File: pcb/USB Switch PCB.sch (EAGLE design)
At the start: 25 parts, among them Q1 2N7002P, Q2 2N7002P, X1 AMPHENOL-0001LF, X2 UE27-USBA

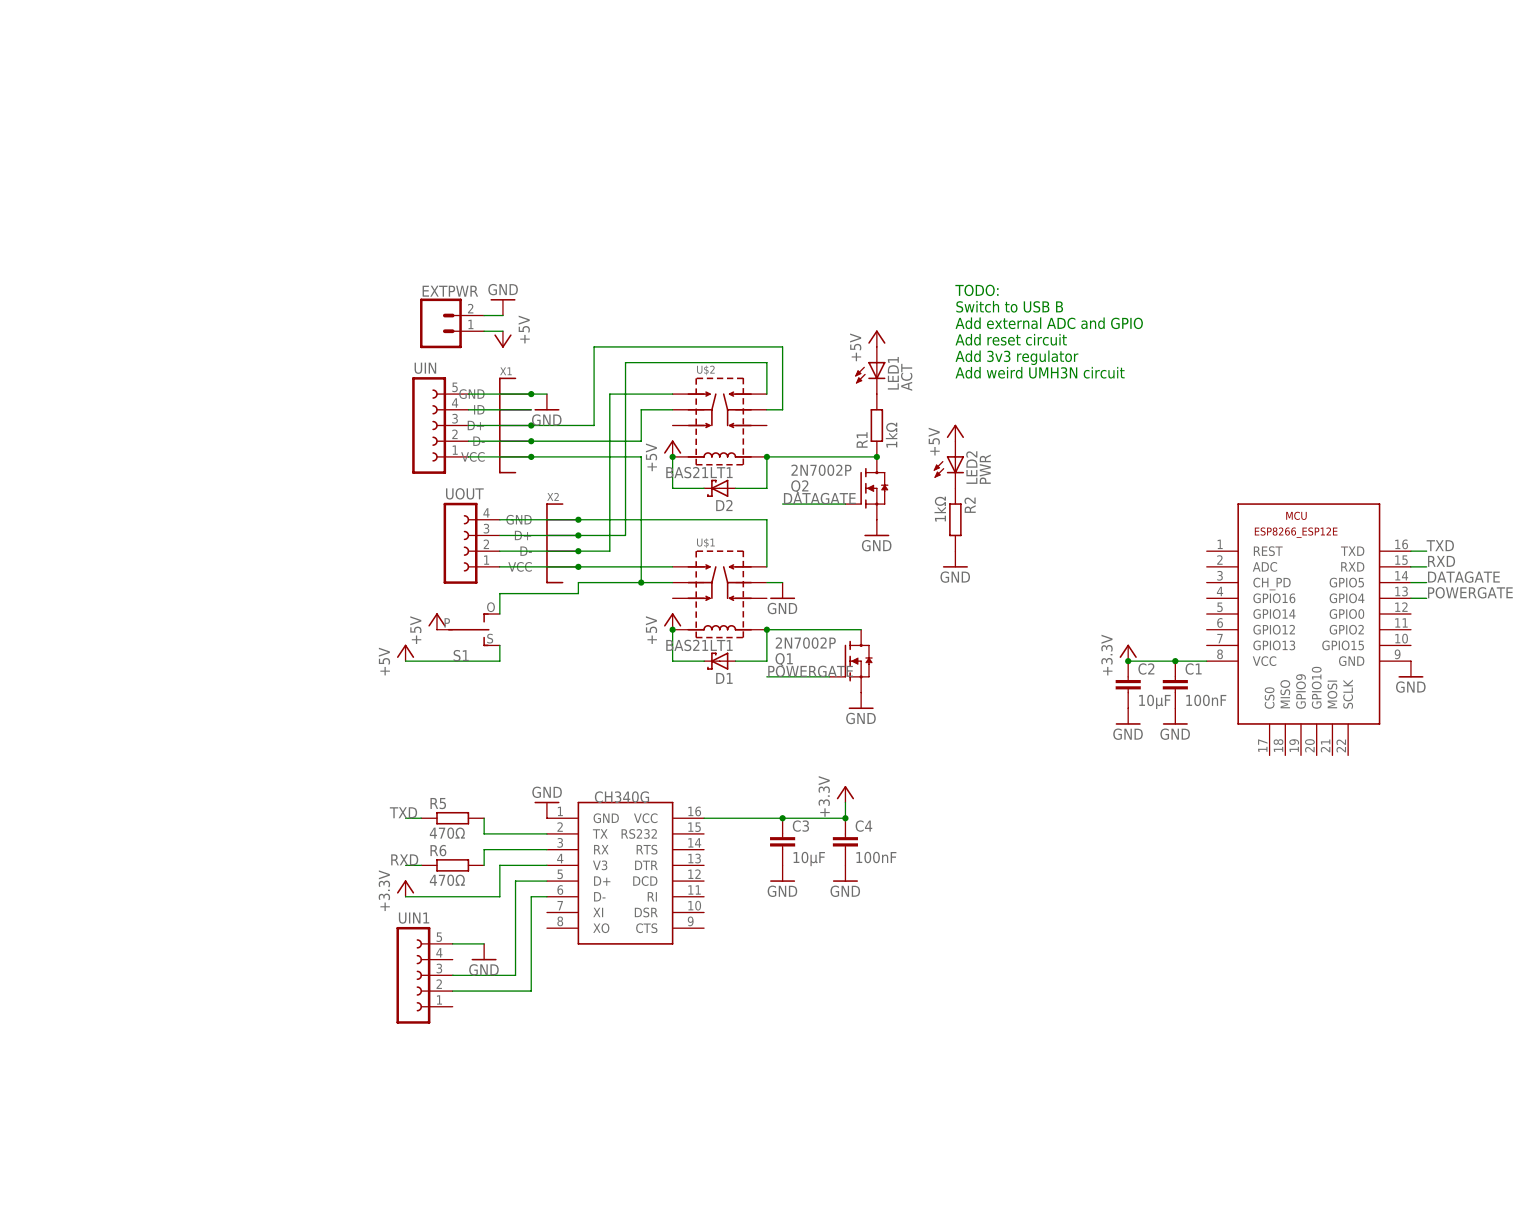
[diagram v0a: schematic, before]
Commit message: More work, looks like shit now.
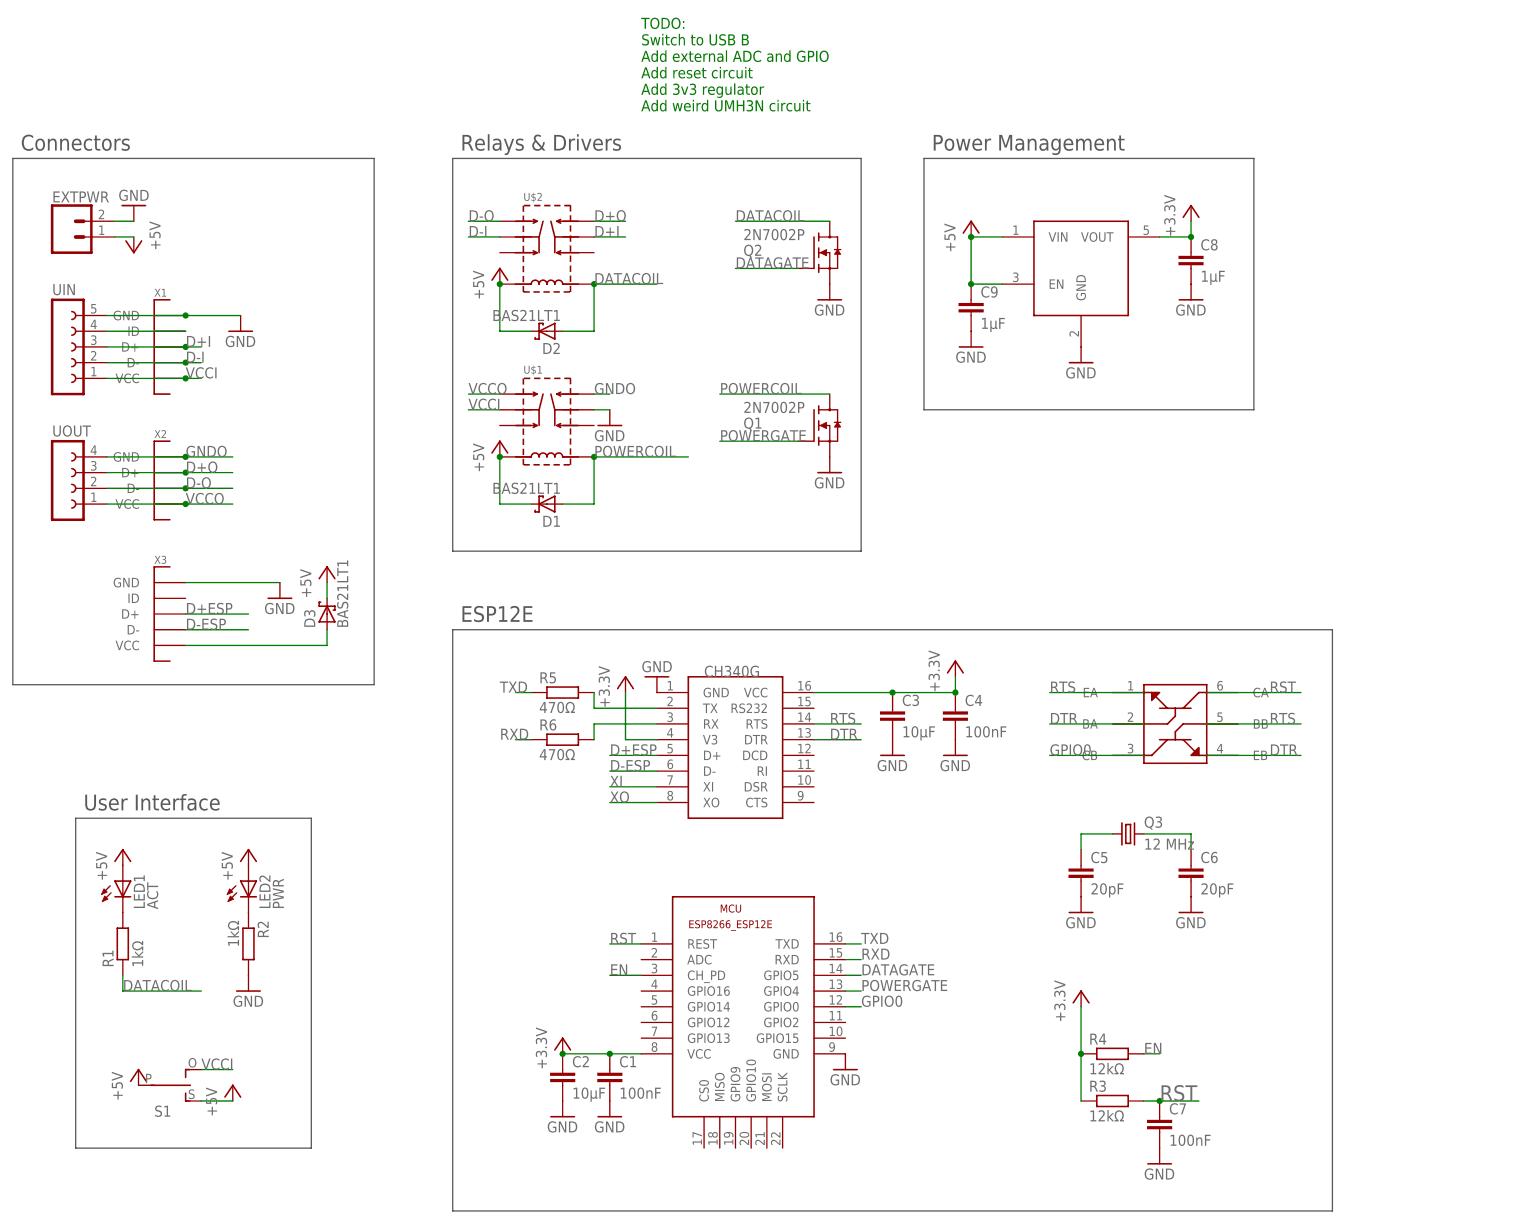
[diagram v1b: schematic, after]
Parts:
- removed UIN1: (no value), USB Switch PCB:FE05-1
- added C5, C6: 20pF, rcl:C-EUC0603
- added C7: 100nF, rcl:C-EUC0603
- added C8, C9: 1µF, rcl:C-EUC0603
- added D3: BAS21LT1, USB Switch PCB:BAS40
- added Q3: 12 MHz, USB Switch PCB:CSM-3XCSM-3X
- added R3, R4: 12kΩ, rcl:R-EU_R0603
- added U$4: UMH3N, USB Switch PCB:UMH3N
- added U$5: MIC5504-3.3YM5SOT23, USB Switch PCB:MIC5504-3.3YM5SOT23
- added X3: AMPHENOL-0001LF, USB Switch PCB:AMPHENOL-0001LF
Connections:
- net 5VUSB renamed VCCI
- net D+ renamed D+I
- net D- renamed D-I
- net N$5 renamed DATACOIL
- net N$6 renamed POWERCOIL
- net VCC0 renamed VCCO
- removed net N$10: U$3.D+, UIN1.3
- removed net N$9: U$3.D-, UIN1.2
- new net D+ESP: U$3.D+, X3.D+
- new net D-ESP: U$3.D-, X3.D-
- new net DTR: U$3.DTR, U$4.BA, U$4.EB
- new net EN: MCU.CH_PD, R4.2
- new net GPIO0: MCU.GPIO0, U$4.CB
- new net N$4: D3.A, X3.VCC
- new net RST: C7.1, MCU.REST, R3.2, U$4.CA
- new net RTS: U$3.RTS, U$4.BB, U$4.EA
- new net XI: C6.1, Q3.2, U$3.XI
- new net XO: C5.1, Q3.1, U$3.XO
- net +5V: now also C8.1, C9.1, D3.C, R3.1, R4.1, U$5.EN, U$5.VIN, U$5.VOUT
- net GND: now also C5.2, C6.2, C7.2, C8.2, C9.2, U$5.GND, X3.GND; no longer UIN1.5
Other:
- note added: "Connectors"
- note added: "ESP12E"
- note added: "Power Management"
- note added: "Relays & Drivers"
- note added: "User Interface"
- moved on the sheet: C1, C2, C3, C4, D1, D2, EXTPWR, LED1, LED2, MCU, Q1, Q2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
